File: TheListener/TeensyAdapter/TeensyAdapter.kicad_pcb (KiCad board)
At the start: 2 copper layers, 19 parts, among them J1 Conn_02x05_Odd_Even, J2 Conn_02x05_Odd_Even, U1 Teensy3.5

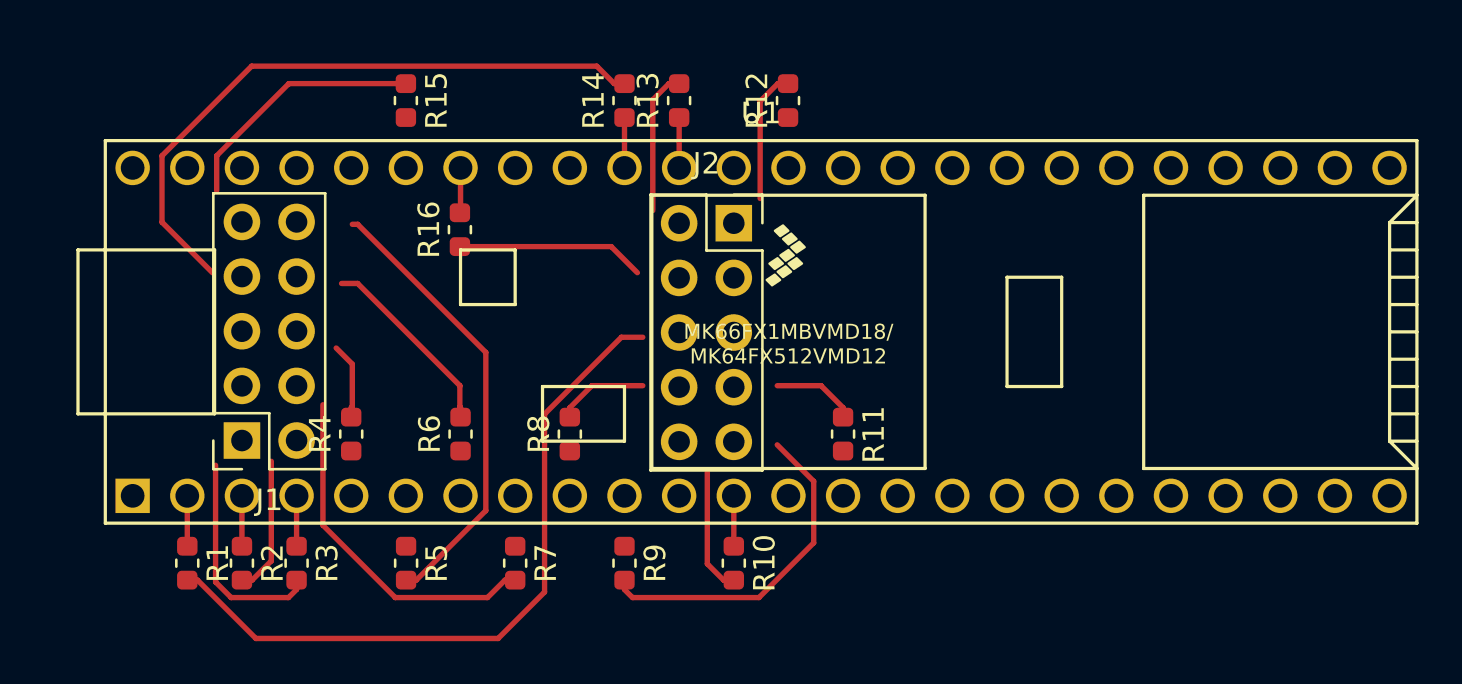
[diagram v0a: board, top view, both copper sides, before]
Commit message: working
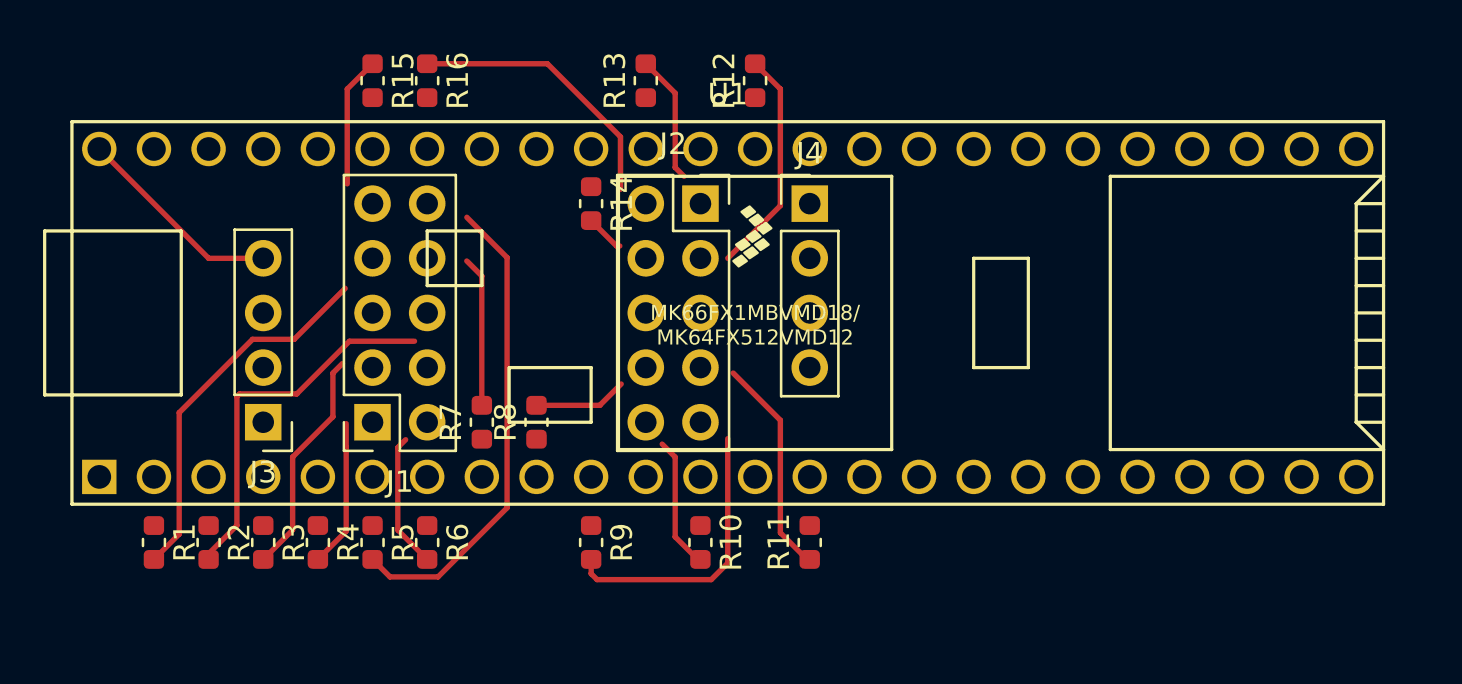
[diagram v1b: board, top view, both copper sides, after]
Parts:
- added J3: Conn_01x04_Male, Connector_PinHeader_2.54mm:PinHeader_1x04_P2.54mm_Vertical, F.Cu at (149.9, 139.7)
- added J4: Conn_01x04_Male, Connector_PinHeader_2.54mm:PinHeader_1x04_P2.54mm_Vertical, F.Cu at (175.3, 129.5)
- moved R16 7.09 mm to (157.5, 123.8), turned to 270 degrees
- moved R7 6.73 mm to (160.0, 139.7), turned to 90 degrees
- moved J1 6.13 mm to (154.9, 139.7)
- moved R11 5.27 mm to (175.3, 145.3), turned to 90 degrees
- moved R6 5.27 mm to (157.5, 145.3), turned to 270 degrees
- moved R4 5.27 mm to (152.4, 145.3), turned to 270 degrees
- moved R14 5.03 mm to (165.1, 129.5), turned to 270 degrees
- moved R5 1.83 mm to (154.9, 145.3)
- moved R1 1.82 mm to (144.8, 145.3)
- moved R2 1.82 mm to (147.3, 145.3)
- moved R9 1.82 mm to (165.1, 145.3)
- moved R10 1.82 mm to (170.2, 145.3)
- moved R3 1.82 mm to (149.9, 145.3)
- moved R13 1.81 mm to (167.6, 123.8)
- moved R15 1.81 mm to (154.9, 123.8)
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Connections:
- J1 pad 1: T_5 -> R_5
- J1 pad 2: R_5 -> T_6
- J1 pad 3: GND -> T_5
- J1 pad 4: T_6 -> R_6
- J1 pad 5: +5V -> (no net)
- J1 pad 6: R_6 -> (no net)
- J2 pad 1: T_1 -> R_1
- J2 pad 2: R_1 -> T_2
- J2 pad 3: GND -> T_1
- J2 pad 4: T_2 -> R_2
- J2 pad 5: +5V -> (no net)
- J2 pad 6: R_2 -> (no net)
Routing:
- net R_6: track 30.0 -> 1.82 mm
- net R_8: track 32.9 -> 17.4 mm
- net R_7: track 6.37 -> 17.4 mm
- net +5V: track 0.00 -> 9.72 mm
- net T_3: track 16.3 -> 6.99 mm
- net R_4: track 3.92 -> 10.3 mm
- net T_8: track 11.8 -> 6.07 mm
- net T_5: track 6.15 -> 10.5 mm
- net T_7: track 8.75 -> 12.8 mm
- net R_1: track 3.54 -> 6.86 mm
- net T_2: track 8.94 -> 6.28 mm
- net T_4: track 15.7 -> 13.1 mm
- net Net-(R3-Pad1): track 2.34 -> 0.00 mm
- net Net-(R2-Pad1): track 2.34 -> 0.00 mm
- net Net-(R14-Pad1): track 2.34 -> 0.00 mm
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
